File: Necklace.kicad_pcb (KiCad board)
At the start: 2 copper layers, 41 x 56.1 mm, 31 parts, among them P1 PICOBLADE_5_HDR_RA, P2 PICOBLADE_5_HDR_RA, SW1 CK_KMR2, U1 ADXL345, U2 MSP430G2452IPW14

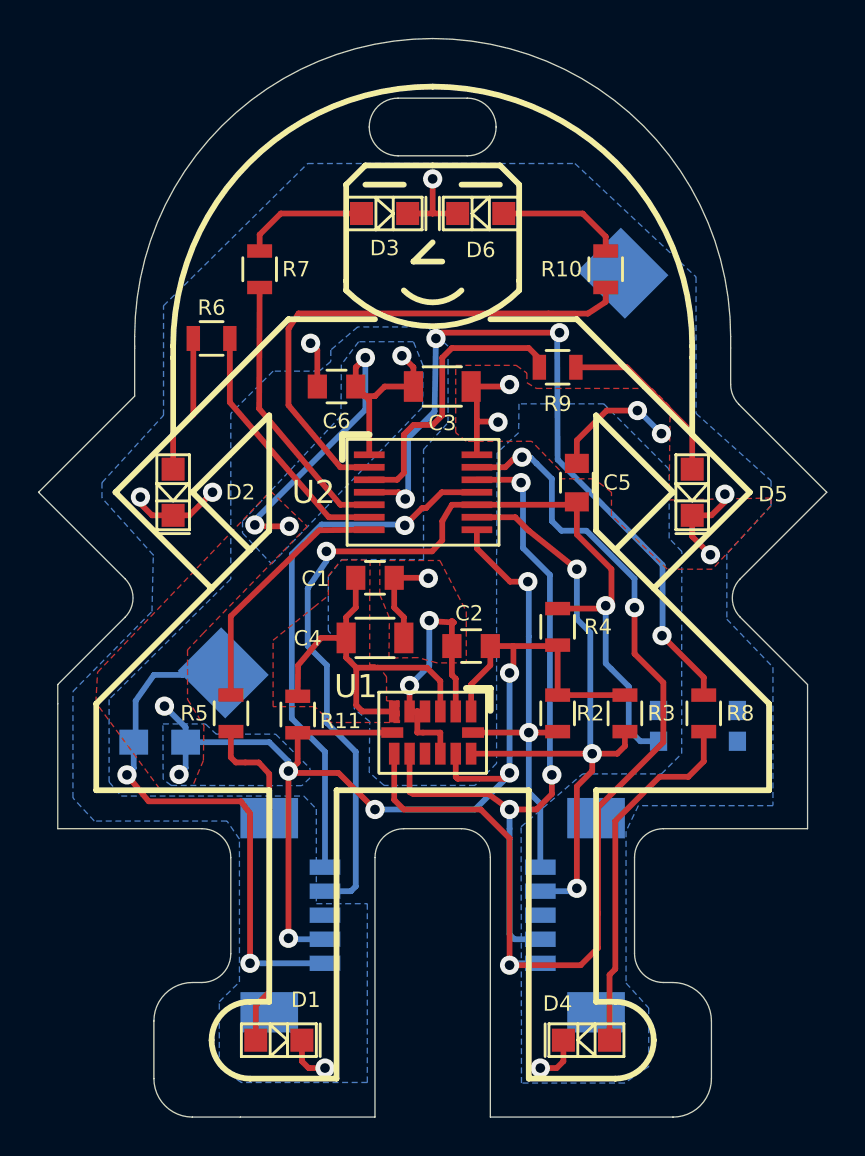
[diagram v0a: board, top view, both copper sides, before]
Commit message: V1.0 ready to fab
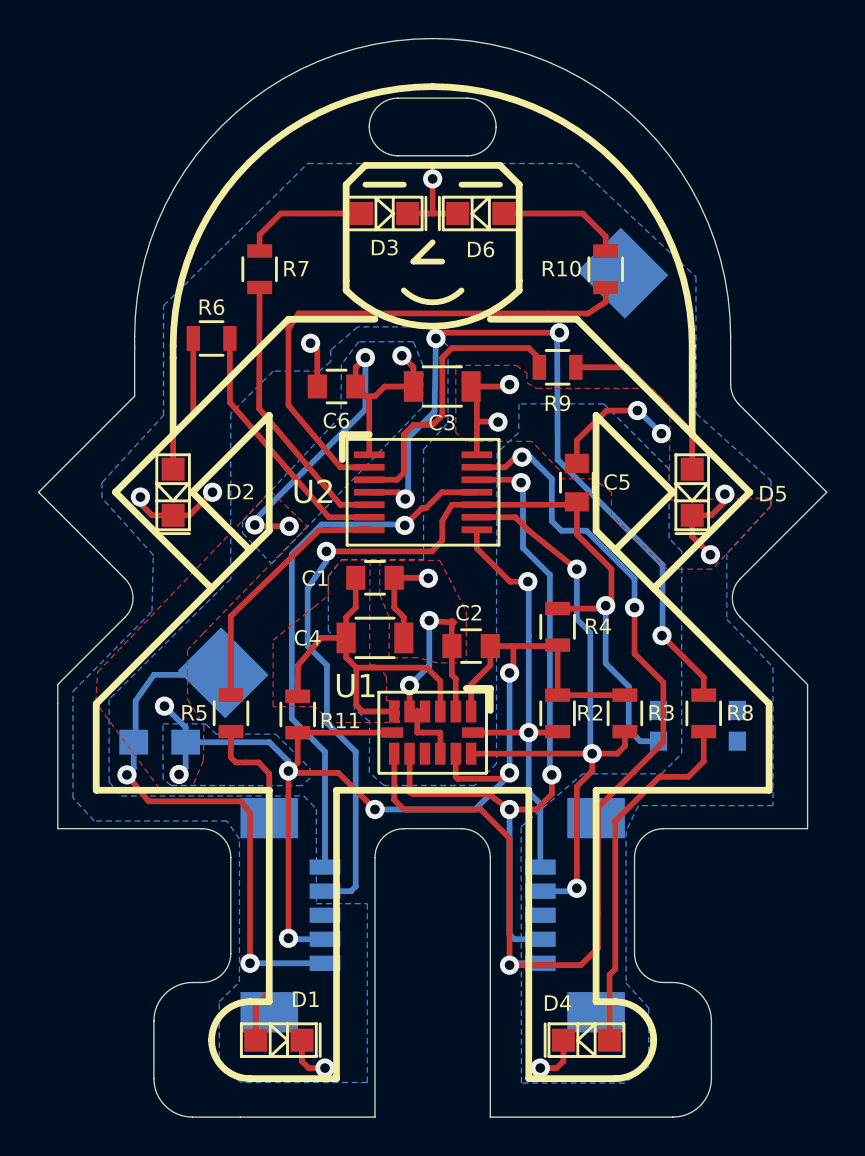
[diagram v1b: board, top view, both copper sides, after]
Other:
- rule via_min_drill: 0.508 -> 0.4
- rule via_min_size: 0.889 -> 0.8
